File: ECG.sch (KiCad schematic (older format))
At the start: 8 parts

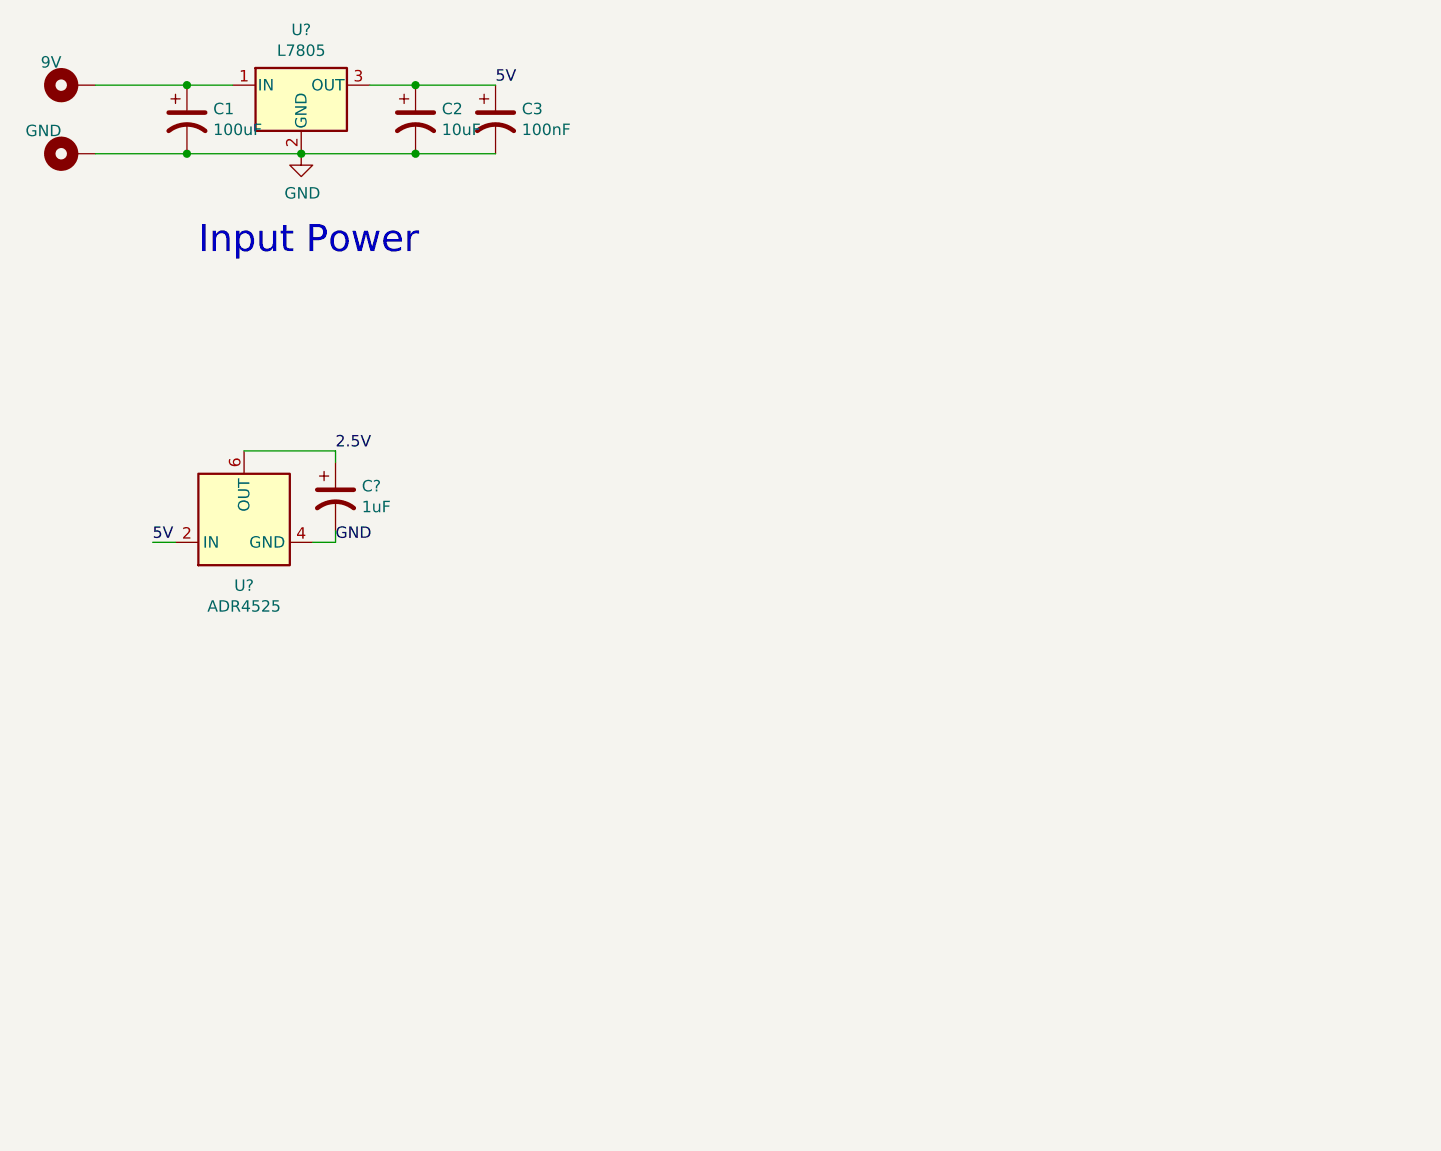
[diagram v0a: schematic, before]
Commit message: Completed power circuits
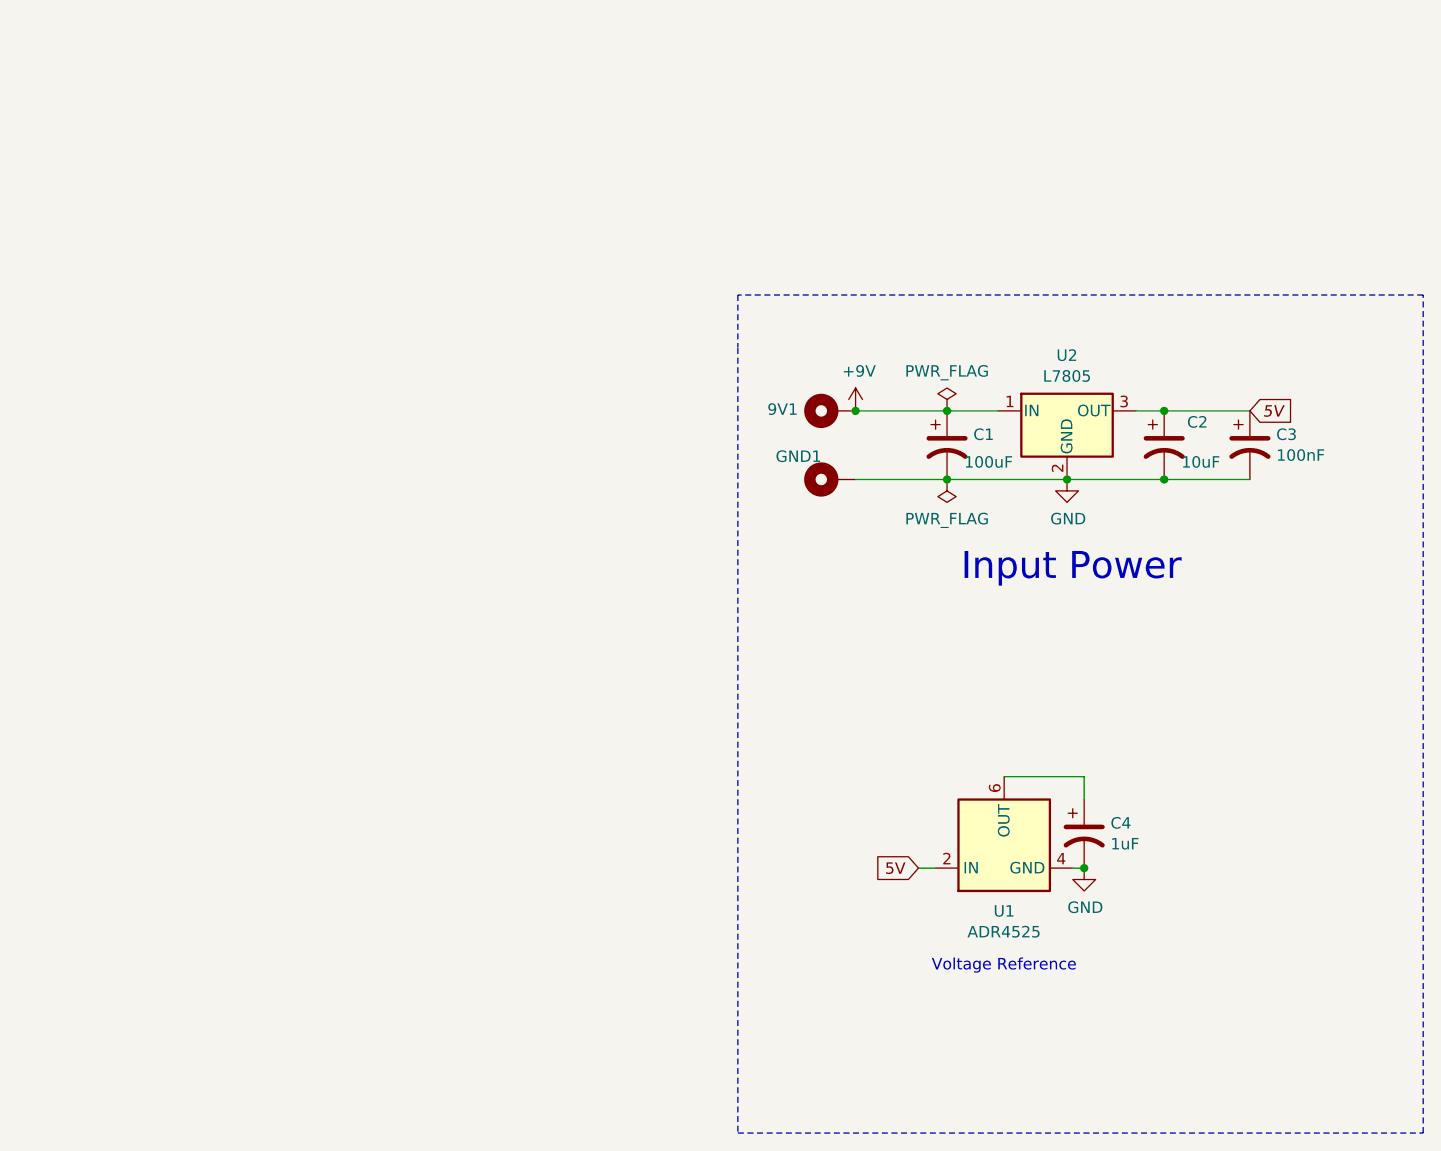
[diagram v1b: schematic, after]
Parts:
- gave numbers to parts that had none: 3
- renumbered 9V to 9V1, GND to GND1
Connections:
- net +9V: now reaches 9V1.1, C1.1, U2.1 (IN)
- net 2.5V: no longer names the net of C4.1, U1.6 (OUT)
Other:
- note added: "Voltage Reference"
- moved on the sheet: 9V1, C1, C2, C3, C4, GND1, U1, U2
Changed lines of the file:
@@
 encoding utf-8
 Sheet 1 1
-Title ""
+Title "Power"
 Date ""
 Rev ""
@@
 $EndDescr
 $Comp
-L Regulator_Linear:L7805 U?
+L Device:CP1 C2
+U 1 1 5F980DB6
+P 5825 2775
+F 0 "C2" H 5925 2875 50  0000 L CNN
+F 1 "10uF" H 5900 2700 50  0000 L CNN
+F 2 "" H 5825 2775 50  0001 C CNN
+F 3 "~" H 5825 2775 50  0001 C CNN
+	1    5825 2775
+	1    0    0    -1
+$EndComp
+$Comp
+L Device:CP1 C3
+U 1 1 5F9833A5
+P 6200 2775
+F 0 "C3" H 6315 2821 50  0000 L CNN
+F 1 "100nF" H 6315 2730 50  0000 L CNN
+F 2 "" H 6200 2775 50  0001 C CNN
+F 3 "~" H 6200 2775 50  0001 C CNN
+	1    6200 2775
+	1    0    0    -1
+$EndComp
+$Comp
+L Mechanical:MountingHole_Pad 9V1
+U 1 1 5F985E28
+P 4375 2625
+F 0 "9V1" V 4381 2777 50  0000 L CNN
+F 1 "MountingHole_Pad" V 4475 2583 50  0001 L CNN
+F 2 "" H 4375 2625 50  0001 C CNN
+F 3 "~" H 4375 2625 50  0001 C CNN
+	1    4375 2625
+	0    -1   -1   0
+$EndComp
+$Comp
+L Mechanical:MountingHole_Pad GND1
+U 1 1 5F98A564
+P 4375 2925
+F 0 "GND1" V 4475 2974 50  0000 L CNN
+F 1 "MountingHole_Pad" V 4475 2883 50  0001 L CNN
+F 2 "" H 4375 2925 50  0001 C CNN
+F 3 "~" H 4375 2925 50  0001 C CNN
+	1    4375 2925
+	0    -1   -1   0
+$EndComp
+Text Notes 4936 3380 0    118  ~ 0
+Input Power
+Text Notes 4808 5084 0    50   ~ 0
+Voltage Reference
+Wire Notes Line
+	3960 2350 3960 5784
+Wire Notes Line
+	3960 5784 6958 5784
+Wire Notes Line
+	6958 5784 6958 2118
+Wire Notes Line
+	6958 2118 3960 2118
+Wire Notes Line
+	3960 2118 3960 2348
+$Comp
+L power:GND #PWR0102
+U 1 1 5F9A88EF
+P 5400 2925
+F 0 "#PWR0102" H 5400 2675 50  0001 C CNN
+F 1 "GND" H 5405 2752 50  0000 C CNN
+F 2 "" H 5400 2925 50  0001 C CNN
+F 3 "" H 5400 2925 50  0001 C CNN
+	1    5400 2925
+	1    0    0    -1
+$EndComp
+$Comp
+L power:+9V #PWR0101
+U 1 1 5F9AB243
+P 4475 2625
+F 0 "#PWR0101" H 4475 2475 50  0001 C CNN
+F 1 "+9V" H 4490 2798 50  0000 C CNN
+F 2 "" H 4475 2625 50  0001 C CNN
+F 3 "" H 4475 2625 50  0001 C CNN
+	1    4475 2625
+	1    0    0    -1
+$EndComp
+$Comp
+L power:PWR_FLAG #FLG01
+U 1 1 5F9B3B5D
+P 4875 2625
+F 0 "#FLG01" H 4875 2700 50  0001 C CNN
+F 1 "PWR_FLAG" H 4875 2798 50  0000 C CNN
+F 2 "" H 4875 2625 50  0001 C CNN
+F 3 "~" H 4875 2625 50  0001 C CNN
+	1    4875 2625
+	1    0    0    -1
+$EndComp
+$Comp
+L Device:CP1 C4
+U 1 1 5F991542
+P 5475 4475
+F 0 "C4" H 5590 4521 50  0000 L CNN
+F 1 "1uF" H 5590 4430 50  0000 L CNN
+F 2 "" H 5475 4475 50  0001 C CNN
+F 3 "~" H 5475 4475 50  0001 C CNN
+	1    5475 4475
+	1    0    0    -1
+$EndComp
+Wire Wire Line
+	4825 4625 4750 4625
+Text GLabel 4750 4625 0    50   Input ~ 0
+5V
+$Comp
+L Reference_Voltage:ADR4525 U1
+U 1 1 5F98E0E5
+P 5125 4525
+F 0 "U1" V 4836 4525 50  0000 C CNN
+F 1 "ADR4525" V 4745 4525 50  0000 C CNN
+F 2 "Package_SO:SOIC-8_3.9x4.9mm_P1.27mm" H 5225 4225 50  0001 C CIN
+F 3 "https://www.analog.com/media/en/technical-documentation/data-sheets/ADR4520_4525_4530_4533_4540_4550.pdf" H 5225 4175 50  0001 C CIN
+	1    5125 4525
+	0    -1   -1   0
+$EndComp
+Wire Wire Line
+	5125 4225 5475 4225
+Wire Wire Line
+	5475 4225 5475 4325
+$Comp
+L power:GND #PWR02
+U 1 1 5F9D2687
+P 5475 4625
+F 0 "#PWR02" H 5475 4375 50  0001 C CNN
+F 1 "GND" H 5480 4452 50  0000 C CNN
+F 2 "" H 5475 4625 50  0001 C CNN
+F 3 "" H 5475 4625 50  0001 C CNN
+	1    5475 4625
+	1    0    0    -1
+$EndComp
+$Comp
+L Regulator_Linear:L7805 U2
 U 1 1 5F977B65
-P 2050 1200
-F 0 "U?" H 2050 1442 50  0000 C CNN
-F 1 "L7805" H 2050 1351 50  0000 C CNN
-F 2 "" H 2075 1050 50  0001 L CIN
-F 3 "http://www.st.com/content/ccc/resource/technical/document/datasheet/41/4f/b3/b0/12/d4/47/88/CD00000444.pdf/files/CD00000444.pdf/jcr:content/translations/en.CD00000444.pdf" H 2050 1150 50  0001 C CNN
-	1    2050 1200
+P 5400 2625
+F 0 "U2" H 5400 2867 50  0000 C CNN
+F 1 "L7805" H 5400 2776 50  0000 C CNN
+F 2 "" H 5425 2475 50  0001 L CIN
+F 3 "http://www.st.com/content/ccc/resource/technical/document/datasheet/41/4f/b3/b0/12/d4/47/88/CD00000444.pdf/files/CD00000444.pdf/jcr:content/translations/en.CD00000444.pdf" H 5400 2575 50  0001 C CNN
+	1    5400 2625
 	1    0    0    -1
 $EndComp
@@
 L Device:CP1 C1
 U 1 1 5F97B8CA
-P 1550 1350
-F 0 "C1" H 1665 1396 50  0000 L CNN
-F 1 "100uF" H 1665 1305 50  0000 L CNN
-F 2 "" H 1550 1350 50  0001 C CNN
-F 3 "~" H 1550 1350 50  0001 C CNN
-	1    1550 1350
-	1    0    0    -1
-$EndComp
-$Comp
-L Device:CP1 C2
-U 1 1 5F980DB6
-P 2550 1350
-F 0 "C2" H 2665 1396 50  0000 L CNN
-F 1 "10uF" H 2665 1305 50  0000 L CNN
-F 2 "" H 2550 1350 50  0001 C CNN
-F 3 "~" H 2550 1350 50  0001 C CNN
-	1    2550 1350
-	1    0    0    -1
-$EndComp
-$Comp
-L Device:CP1 C3
-U 1 1 5F9833A5
-P 2900 1350
-F 0 "C3" H 3015 1396 50  0000 L CNN
-F 1 "100nF" H 3015 1305 50  0000 L CNN
-F 2 "" H 2900 1350 50  0001 C CNN
-F 3 "~" H 2900 1350 50  0001 C CNN
-	1    2900 1350
-	1    0    0    -1
-$EndComp
-$Comp
-L power:GND #PWR?
-U 1 1 5F983C07
-P 2050 1500
-F 0 "#PWR?" H 2050 1250 50  0001 C CNN
-F 1 "GND" H 2055 1327 50  0000 C CNN
-F 2 "" H 2050 1500 50  0001 C CNN
-F 3 "" H 2050 1500 50  0001 C CNN
-	1    2050 1500
-	1    0    0    -1
-$EndComp
-Wire Wire Line
-	1550 1500 2050 1500
-Connection ~ 2050 1500
-Wire Wire Line
-	2900 1500 2550 1500
-Wire Wire Line
-	2050 1500 2550 1500
-Connection ~ 2550 1500
-Wire Wire Line
-	1550 1200 1750 1200
-Wire Wire Line
-	2350 1200 2550 1200
-Wire Wire Line
-	2900 1200 2550 1200
-Connection ~ 2550 1200
-$Comp
-L Mechanical:MountingHole_Pad 9V
-U 1 1 5F985E28
-P 1050 1200
-F 0 "9V" V 1150 1249 50  0000 L CNN
-F 1 "MountingHole_Pad" V 1150 1158 50  0001 L CNN
-F 2 "" H 1050 1200 50  0001 C CNN
-F 3 "~" H 1050 1200 50  0001 C CNN
-	1    1050 1200
-	0    -1   -1   0
-$EndComp
-$Comp
-L Mechanical:MountingHole_Pad GND
-U 1 1 5F98A564
-P 1050 1500
-F 0 "GND" V 1150 1549 50  0000 L CNN
-F 1 "MountingHole_Pad" V 1150 1458 50  0001 L CNN
-F 2 "" H 1050 1500 50  0001 C CNN
-F 3 "~" H 1050 1500 50  0001 C CNN
-	1    1050 1500
-	0    -1   -1   0
-$EndComp
-Wire Wire Line
-	1150 1200 1550 1200
-Connection ~ 1550 1200
-Wire Wire Line
-	1550 1500 1150 1500
-Connection ~ 1550 1500
-Text Label 2900 1200 0    50   ~ 0
+P 4875 2775
+F 0 "C1" H 4990 2821 50  0000 L CNN
+F 1 "100uF" H 4950 2700 50  0000 L CNN
+F 2 "" H 4875 2775 50  0001 C CNN
+F 3 "~" H 4875 2775 50  0001 C CNN
+	1    4875 2775
+	1    0    0    -1
+$EndComp
+Wire Wire Line
+	4475 2925 4875 2925
+Connection ~ 4875 2925
+Wire Wire Line
+	5400 2925 4875 2925
+Connection ~ 5400 2925
+Wire Wire Line
+	4875 2625 4475 2625
+Connection ~ 4875 2625
+Connection ~ 4475 2625
+Wire Wire Line
+	4875 2625 5100 2625
+Wire Wire Line
+	5700 2625 5825 2625
+Wire Wire Line
+	5400 2925 5825 2925
+Wire Wire Line
+	6200 2925 5825 2925
+Connection ~ 5825 2925
+Wire Wire Line
+	6200 2625 5825 2625
+Connection ~ 5825 2625
+Text GLabel 6200 2625 2    50   Input Italic 0
 5V
-Text Notes 1600 1950 0    118  ~ 0
-Input Power
-$Comp
-L Reference_Voltage:ADR4525 U?
-U 1 1 5F98E0E5
-P 1800 3100
-F 0 "U?" V 1511 3100 50  0000 C CNN
-F 1 "ADR4525" V 1420 3100 50  0000 C CNN
-F 2 "Package_SO:SOIC-8_3.9x4.9mm_P1.27mm" H 1900 2800 50  0001 C CIN
-F 3 "https://www.analog.com/media/en/technical-documentation/data-sheets/ADR4520_4525_4530_4533_4540_4550.pdf" H 1900 2750 50  0001 C CIN
-	1    1800 3100
-	0    -1   -1   0
-$EndComp
-Text Label 1400 3200 0    50   ~ 0
-5V
-Wire Wire Line
-	1400 3200 1500 3200
-Text Label 2200 3200 0    50   ~ 0
-GND
-Wire Wire Line
-	2100 3200 2200 3200
-$Comp
-L Device:CP1 C?
-U 1 1 5F991542
-P 2200 3000
-F 0 "C?" H 2315 3046 50  0000 L CNN
-F 1 "1uF" H 2315 2955 50  0000 L CNN
-F 2 "" H 2200 3000 50  0001 C CNN
-F 3 "~" H 2200 3000 50  0001 C CNN
-	1    2200 3000
-	1    0    0    -1
-$EndComp
-Wire Wire Line
-	2200 3150 2200 3200
-Wire Wire Line
-	1800 2800 2200 2800
-Wire Wire Line
-	2200 2800 2200 2850
-Text Label 2200 2800 0    50   ~ 0
-2.5V
+Wire Wire Line
+	5425 4625 5475 4625
+Connection ~ 5475 4625
+$Comp
+L power:PWR_FLAG #FLG?
+U 1 1 5F9F7887
+P 4875 2925
+F 0 "#FLG?" H 4875 3000 50  0001 C CNN
+F 1 "PWR_FLAG" H 4875 3098 50  0000 C CNN
+F 2 "" H 4875 2925 50  0001 C CNN
+F 3 "~" H 4875 2925 50  0001 C CNN
+	1    4875 2925
+	-1   0    0    1
+$EndComp
 $EndSCHEMATC
